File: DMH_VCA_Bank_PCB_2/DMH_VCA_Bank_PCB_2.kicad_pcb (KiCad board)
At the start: 2 copper layers, 48 x 108 mm, 17 parts, among them J0 Conn_01x01, J50 Conn_01x06, J60 Conn_01x06, J70 Conn_01x06, J80 Conn_01x06

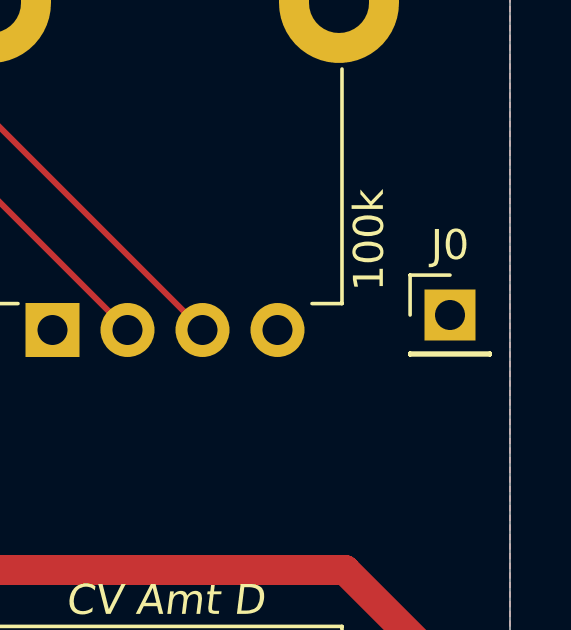
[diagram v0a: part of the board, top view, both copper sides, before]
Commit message: KiCad 10 and updated SynthStuff
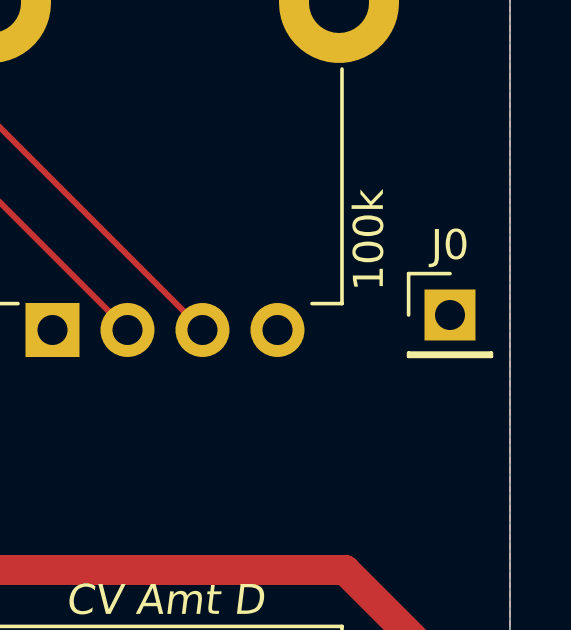
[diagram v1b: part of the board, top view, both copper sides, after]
